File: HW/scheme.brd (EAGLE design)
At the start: 16.5 x 28 mm, 7 parts, among them IC1 FT245RL

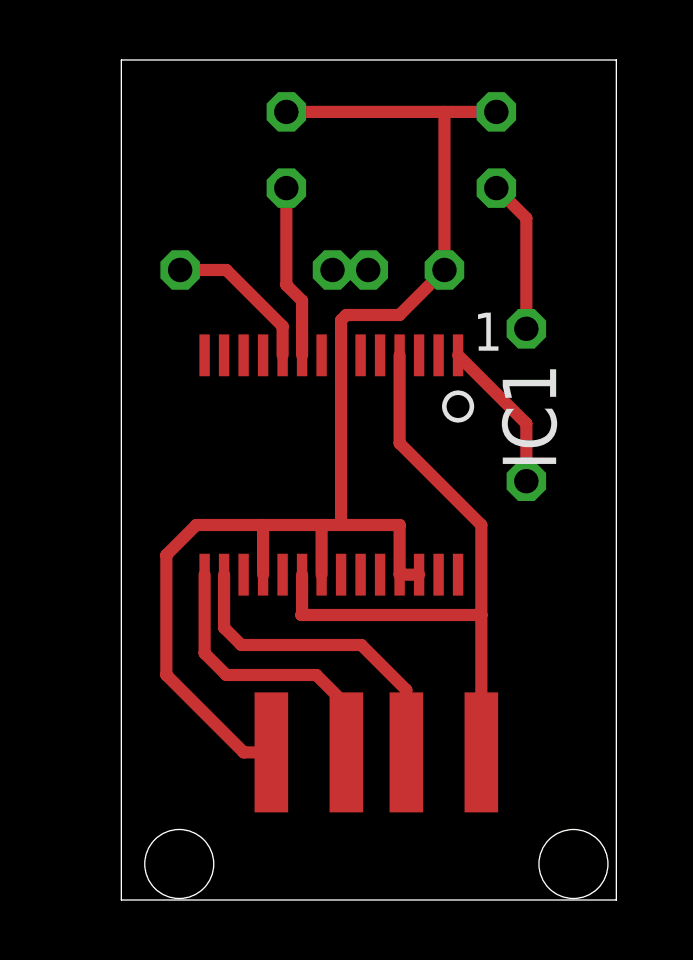
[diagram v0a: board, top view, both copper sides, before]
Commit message: Board v2
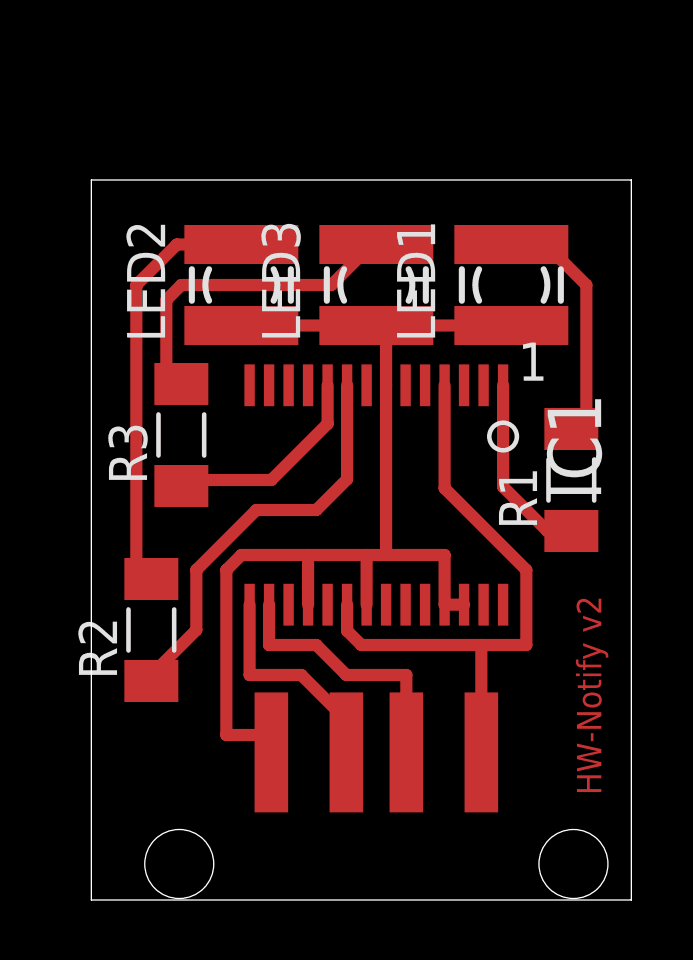
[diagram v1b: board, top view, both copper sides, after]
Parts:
- added R3: 130, resistor:M1406
- LED1, LED2: device led:LED5MM -> led:NFSG036BT
- LED3: device led:LED3MM -> led:NFSG036BT
- R1: value (none) -> 330; device resistor:0204/5 -> resistor:M1406
- R2: value (none) -> 150; device resistor:0204/5 -> resistor:M1406
- moved R2 12.5 mm to (0.00, 9.00), flipped to the top, turned to 90 degrees
- moved LED2 4.74 mm to (3.00, 20.5), flipped to the top
- moved LED1 4.53 mm to (12.0, 20.5), flipped to the top
- moved R1 2.92 mm to (14.0, 14.0), flipped to the top
- moved IC1 1.80 mm to (7.50, 13.5)
- moved LED3 1.12 mm to (7.50, 20.5), flipped to the top, turned to 90 degrees
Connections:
- new net N$9: LED3.A, R3.2
- net GND: now also LED1.C, LED2.C, LED3.C; no longer LED1.K, LED2.K, LED3.K
- net N$5: now also R3.1; no longer R2.1
- net N$6: now also R2.1; no longer LED2.A
- net N$7: now also LED2.A; no longer LED3.A
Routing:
- net N$7: track 1.19 -> 14.1 mm
- net N$9: track 0.00 -> 10.8 mm
- net GND: track 45.7 -> 37.7 mm
- net N$6: track 5.79 -> 13.7 mm
- net N$8: track 5.10 -> 8.07 mm
- net N$3: track 9.64 -> 7.27 mm
- net N$2: track 10.8 -> 8.91 mm
- net N$5: track 5.16 -> 7.02 mm
- net N$1: track 21.7 -> 20.4 mm
- net N$4: track 5.14 -> 6.27 mm
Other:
- board size 16.5 x 28 mm -> 18 x 24 mm
- board text added: "HW-Notify v2"
